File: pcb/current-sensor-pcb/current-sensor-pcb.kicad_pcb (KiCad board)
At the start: 2 copper layers, 12 parts, among them U1 TLI4971A050T5UE0001XUMA1

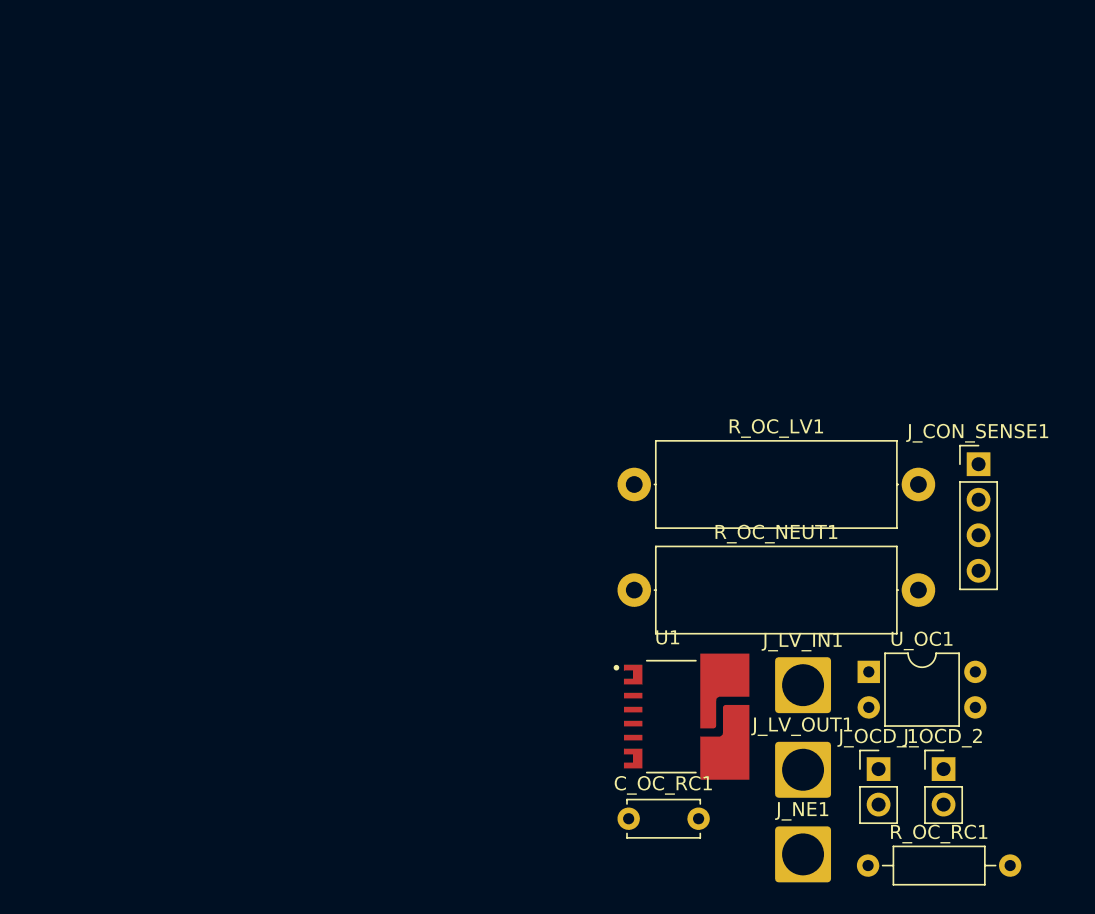
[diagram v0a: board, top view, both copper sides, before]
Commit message: Progress with SMT controller and contactor variant
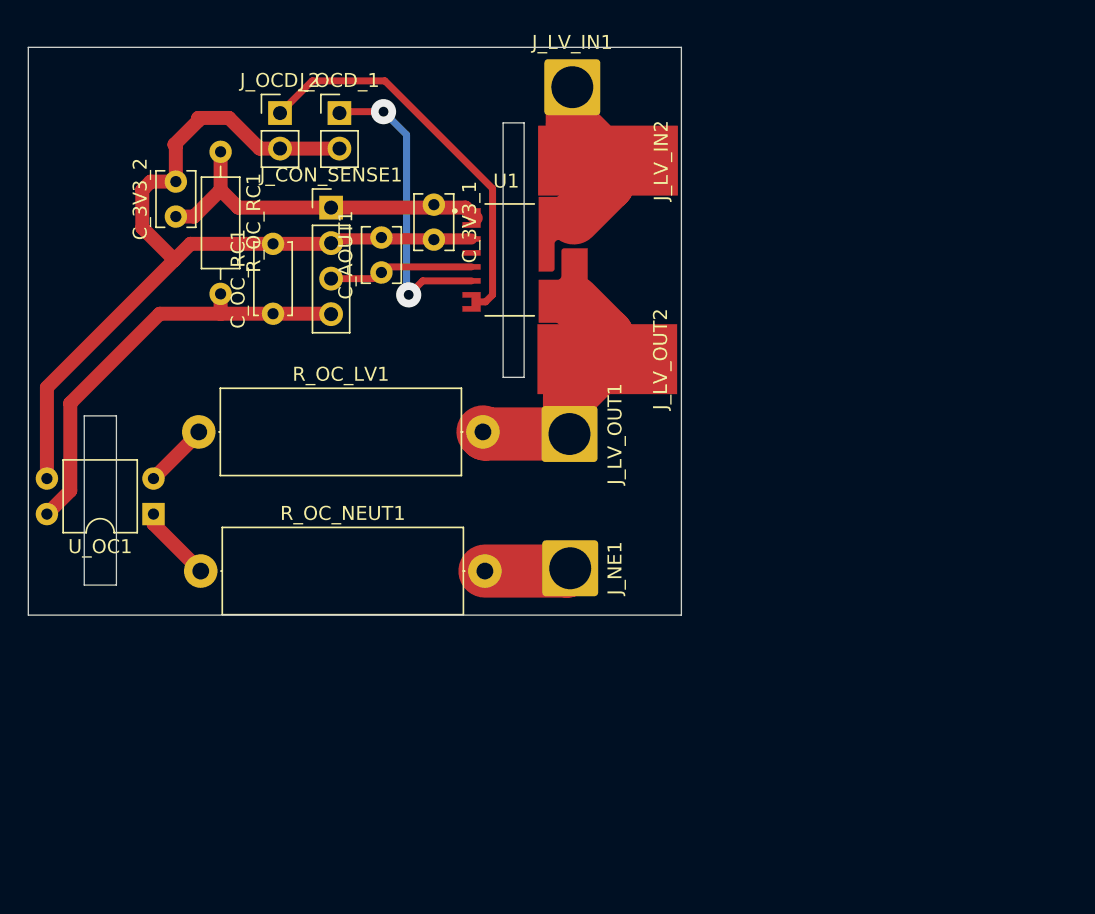
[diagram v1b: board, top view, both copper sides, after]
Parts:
- added C_3V3_1: C, Capacitor_THT:C_Disc_D3.8mm_W2.6mm_P2.50mm, F.Cu at (28.9, 11.2)
- added C_3V3_2: C, Capacitor_THT:C_Disc_D3.8mm_W2.6mm_P2.50mm, F.Cu at (10.4, 12.0)
- added C_AOUT1: C, Capacitor_THT:C_Disc_D3.8mm_W2.6mm_P2.50mm, F.Cu at (25.1, 16.0)
- added J_LV_IN2: Conn_01x01_Socket, Connector_Wire:SolderWirePad_1x01_SMD_5x10mm, F.Cu at (41.4, 8.00)
- added J_LV_OUT2: Conn_01x01_Socket, Connector_Wire:SolderWirePad_1x01_SMD_5x10mm, F.Cu at (41.3, 22.2)
- moved R_OC_RC1 68.9 mm to (13.7, 7.37), turned to -90 degrees
- moved J_OCD_2 66.7 mm to (17.9, 4.60)
- moved J_OCD_1 60.7 mm to (22.1, 4.60)
- moved U_OC1 52.4 mm to (8.85, 33.3), turned to 180 degrees
- moved J_CON_SENSE1 49.8 mm to (21.6, 11.4)
- moved J_LV_IN1 45.8 mm to (38.8, 2.75)
- moved C_OC_RC1 44.2 mm to (17.4, 18.9), turned to 90 degrees
- moved U1 34.6 mm to (35.4, 15.1)
- moved R_OC_LV1 31.4 mm to (12.1, 27.4)
- moved R_OC_NEUT1 31.0 mm to (12.2, 37.4)
- moved J_LV_OUT1 29.2 mm to (38.6, 27.6), turned to -90 degrees
- moved J_NE1 26.4 mm to (38.6, 37.1), turned to -90 degrees
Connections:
- U_OC1 pad 1: Net-(R_OC_LV1-Pad1) -> Net-(R_OC_NEUT1-Pad1)
- U_OC1 pad 2: Net-(R_OC_NEUT1-Pad1) -> Net-(R_OC_LV1-Pad1)
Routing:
- net GND: track 0.00 -> 66.2 mm
- net Net-(J_CON_SENSE1-Pin_4): track 0.00 -> 31.4 mm
- net Net-(J_OCD_2-Pin_1): track 0.00 -> 28.3 mm
- net +3V3: track 0.00 -> 25.8 mm
- net Net-(J_OCD_1-Pin_1): track 0.00 -> 22.0 mm, vias 0 -> 2
- net Net-(J_LV_OUT1-Pin_1): track 0.00 -> 17.8 mm
- net Net-(J_LV_IN1-Pin_1): track 0.00 -> 11.4 mm
- net Net-(J_CON_SENSE1-Pin_3): track 0.00 -> 10.4 mm
- net Net-(J_NE1-Pin_1): track 0.00 -> 6.18 mm
- net Net-(R_OC_NEUT1-Pad1): track 0.00 -> 5.48 mm
- net Net-(R_OC_LV1-Pad1): track 0.00 -> 4.68 mm
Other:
- board outline added: 46.7 x 40.6 mm
